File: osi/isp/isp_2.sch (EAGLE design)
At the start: 2 parts

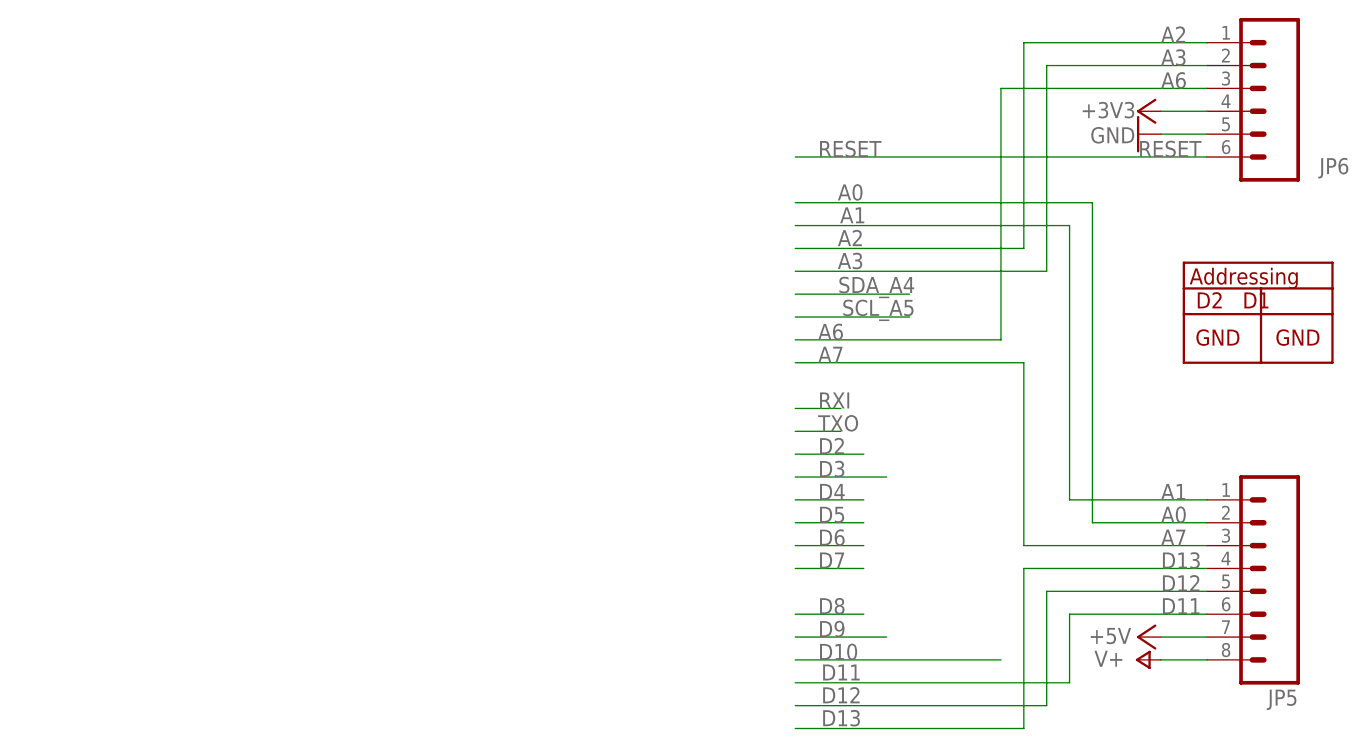
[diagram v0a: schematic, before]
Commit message: layout changes
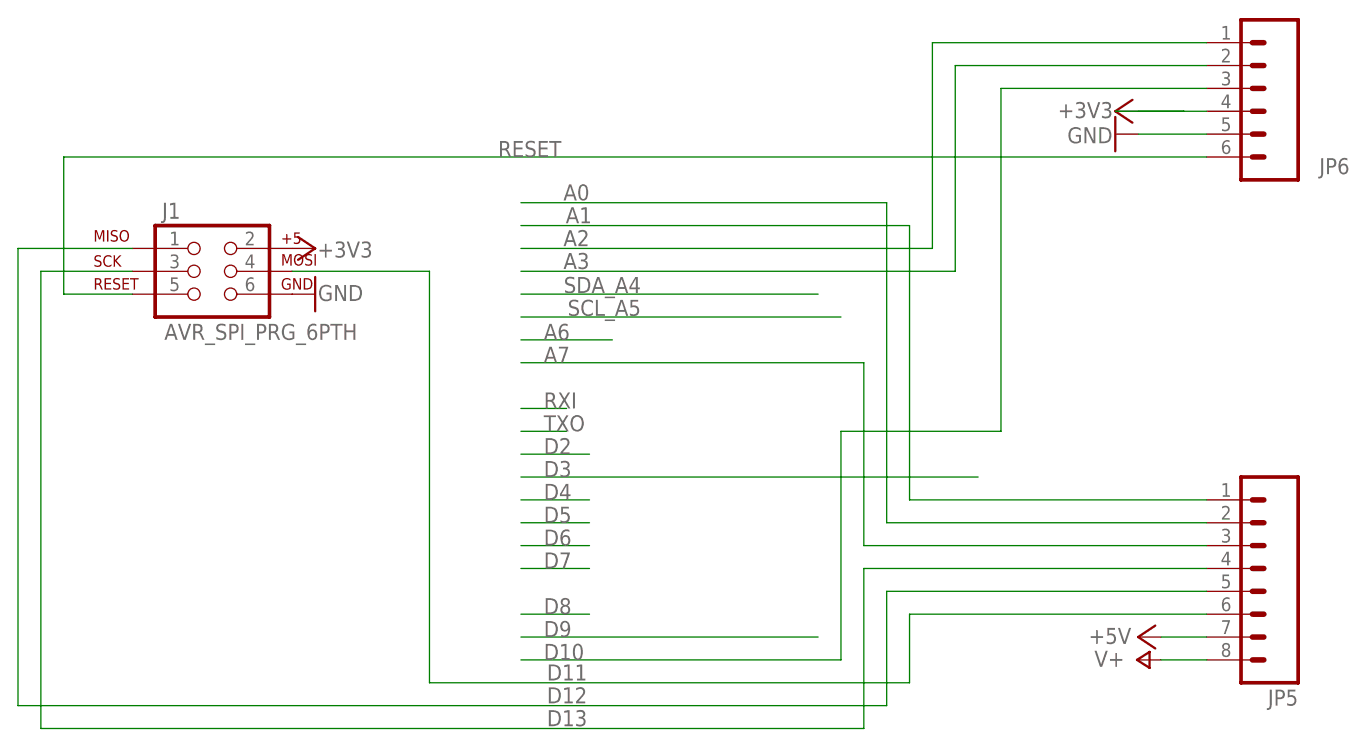
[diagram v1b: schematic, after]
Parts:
- added J1: AVR_SPI_PRG_6PTH, SparkFun:AVR_SPI_PRG_6PTH
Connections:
- net A6 renamed D10
- net +3V3: now also J1.2
- net D11: now also J1.4
- net D12: now also J1.1
- net D13: now also J1.3
- net GND: now also J1.6
- net RESET: now also J1.5
